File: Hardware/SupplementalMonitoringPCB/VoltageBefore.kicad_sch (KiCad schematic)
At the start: 7 parts, among them IC1 TLV9002QDRQ1

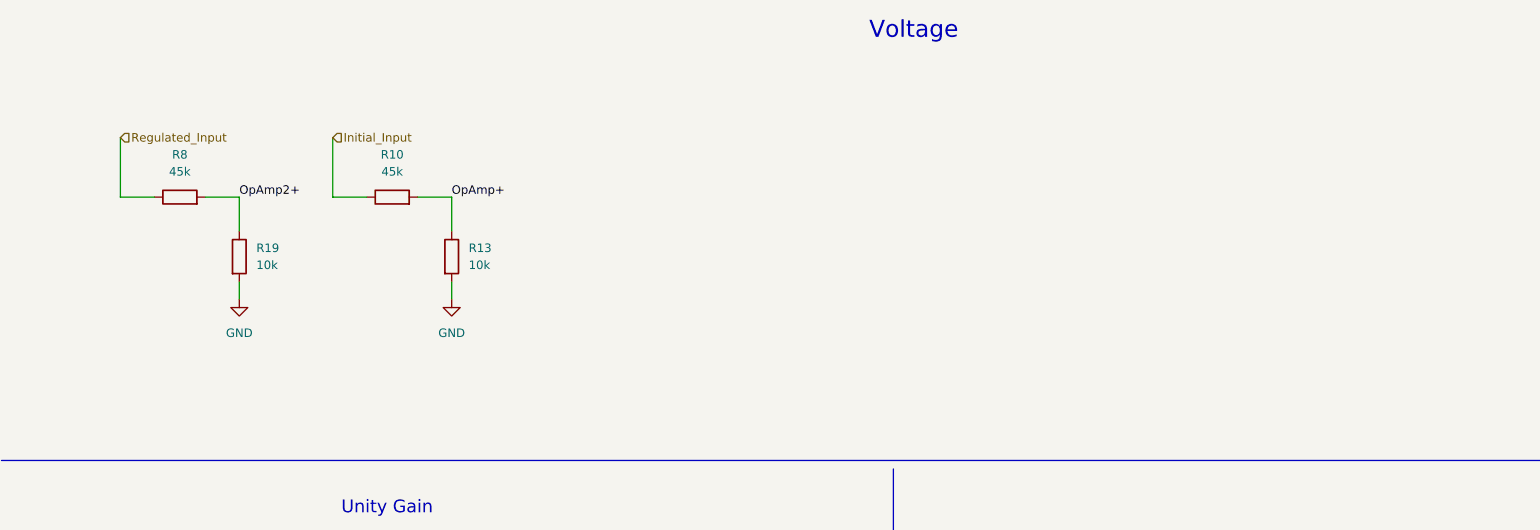
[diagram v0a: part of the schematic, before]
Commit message: 9/27 Workday
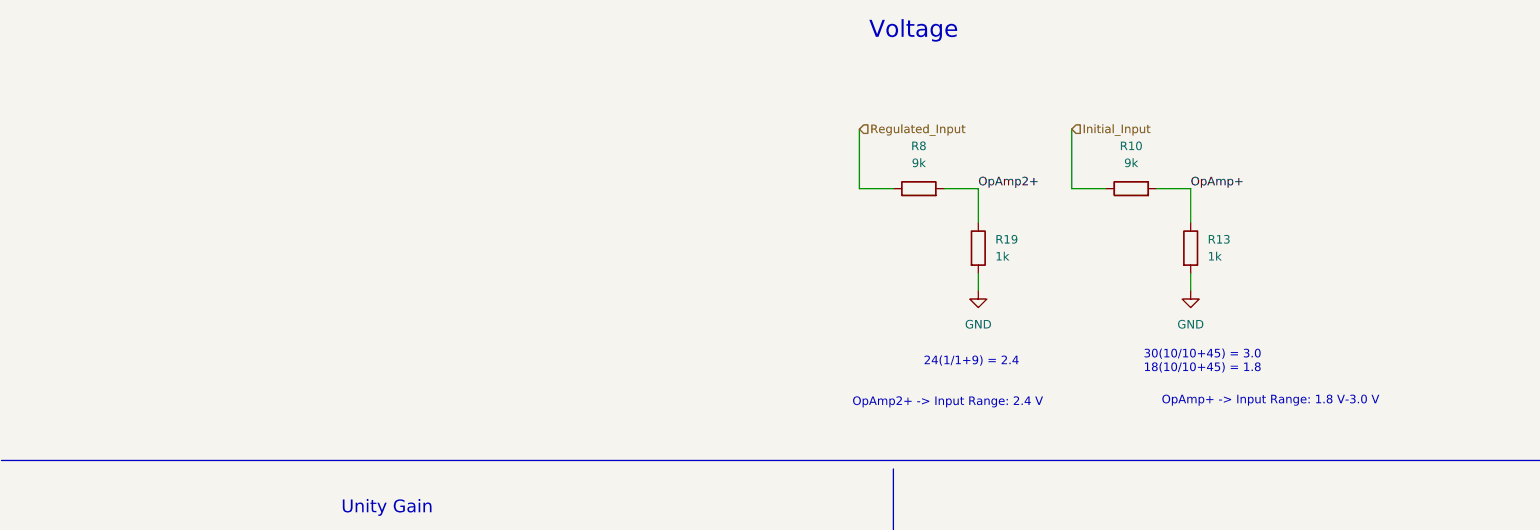
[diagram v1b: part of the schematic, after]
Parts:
- R10, R8: value 45k -> 9k
- R13, R19: value 10k -> 1k
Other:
- note added: "24(1/1+9) = 2.4"
- note added: "30(10/10+45) = 3.0 18(10/10+45) = 1.8"
- note added: "OpAmp+ -> Input Range: 1.8 V-3.0 V"
- note added: "OpAmp2+ -> Input Range: 2.4 V"
- moved on the sheet: R10, R13, R19, R8
